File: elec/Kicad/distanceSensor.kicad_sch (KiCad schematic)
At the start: 14 parts, among them J4 Conn_01x05, Q2 BSS138, Q3 BSS138, U5 VL53L0CXV0DH1, U6 MIC5219-2.8YM5

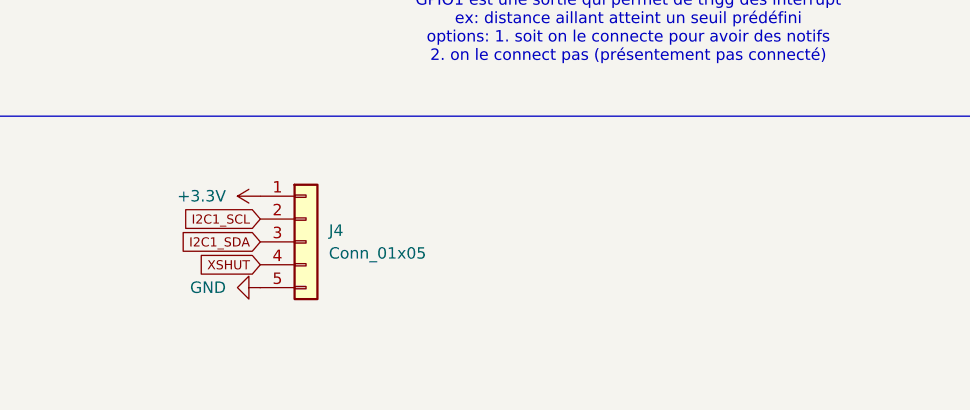
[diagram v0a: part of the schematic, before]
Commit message: sorry Jacob tu va être dessus ...
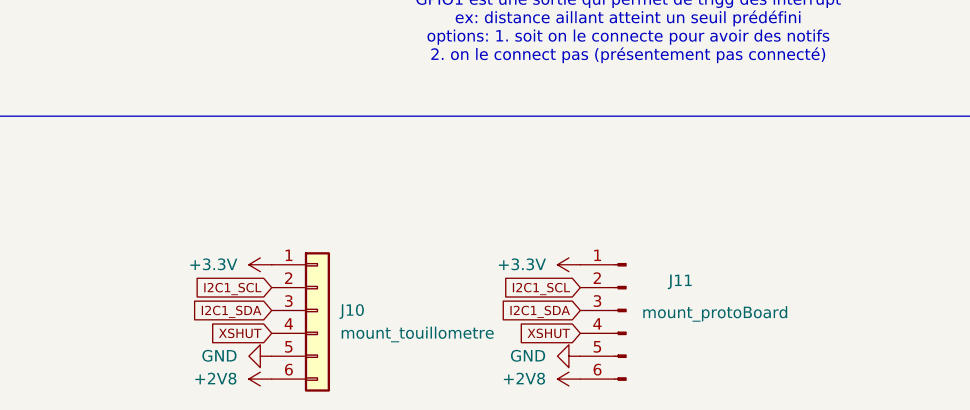
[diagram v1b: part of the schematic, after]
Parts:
- removed J4: Conn_01x05, Connector_PinSocket_2.54mm:PinSocket_1x05_P2.54mm_Vertical, symbol Connector_Generic:Conn_01x05
- added J10: mount_touillometre, Connector_PinSocket_2.54mm:PinSocket_1x06_P2.54mm_Vertical, symbol Connector_Generic:Conn_01x06
- added J11: mount_protoBoard, Connector_PinSocket_2.54mm:PinSocket_1x06_P2.54mm_Vertical, symbol Connector:Conn_01x06_Pin
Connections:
- net +2V8: now also J10.6 (Pin_6), J11.6 (Pin_6)
- net +3.3V: now also J10.1 (Pin_1), J11.1 (Pin_1)
- net GND: now also J10.5 (Pin_5), J11.5 (Pin_5)
- net I2C1_SCL: now also J10.2 (Pin_2), J11.2 (Pin_2)
- net I2C1_SDA: now also J10.3 (Pin_3), J11.3 (Pin_3)
- net XSHUT: now also J10.4 (Pin_4), J11.4 (Pin_4)
